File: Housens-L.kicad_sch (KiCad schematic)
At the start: 37 parts, among them J1 JTAG/SWD, J2 USB_C_2.0, SW1 RESET, U1 MCP1603, U2 BME280, U3 OPT3005, U4 STM32WB55CGUx, Y1 32MHz, Y2 32.768kHz

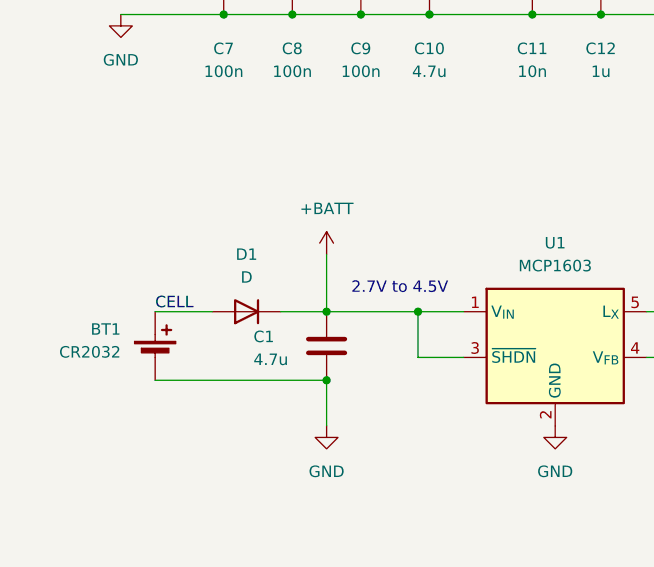
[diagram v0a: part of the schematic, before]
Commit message: Layout antenna
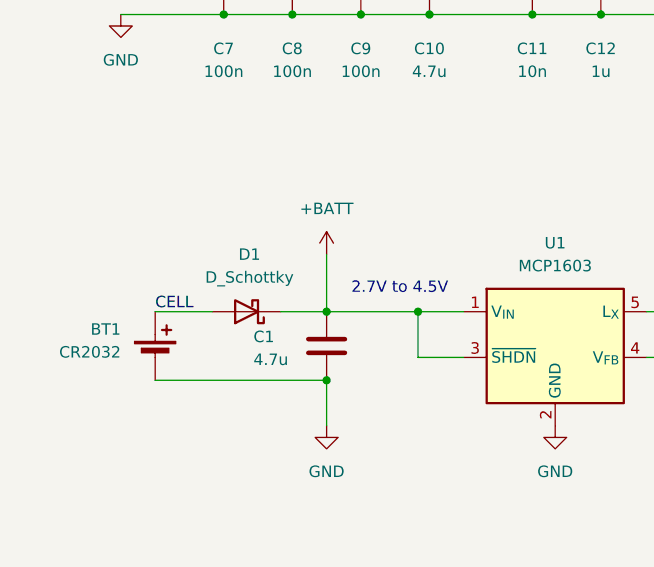
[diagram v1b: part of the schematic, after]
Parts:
- removed D1: D, Diode_SMD:D_0603_1608Metric, symbol Device:D
- added D1: D_Schottky, Diode_SMD:D_0603_1608Metric, symbol Device:D_Schottky
- Y1, Y2: footprint (none) -> Crystal:Crystal_SMD_2520-4Pin_2.5x2.0mm
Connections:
- net +BATT: now also D1.1 (K)
- net CELL: now also D1.2 (A)
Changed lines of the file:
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@@
+	)
+	(symbol
+		(lib_id "Device:D_Schottky")
+		(at 40.64 170.18 180)
+		(unit 1)
+		(exclude_from_sim no)
+		(in_bom yes)
+		(on_board yes)
+		(dnp no)
+		(fields_autoplaced yes)
+		(property "Reference" "D1"
+			(at 40.9575 163.83 0)
+			(effects
+				(font
+					(size 1.27 1.27)
+				)
+			)
+		)
+		(property "Value" "D_Schottky"
+			(at 40.9575 166.37 0)
+			(effects
+				(font
+					(size 1.27 1.27)
+				)
+			)
+		)
+		(property "Footprint" "Diode_SMD:D_0603_1608Metric"
+			(at 40.64 170.18 0)
+			(effects
+				(font
+					(size 1.27 1.27)
+				)
+				(hide yes)
+			)
+		)
+		(property "Datasheet" "~"
+			(at 40.64 170.18 0)
+			(effects
+				(font
+					(size 1.27 1.27)
+				)
+				(hide yes)
+			)
+		)
+		(property "Description" "Schottky diode"
+			(at 40.64 170.18 0)
+			(effects
+				(font
+					(size 1.27 1.27)
+				)
+				(hide yes)
+			)
+		)
+		(pin "2"
+		)
+		(pin "1"
+		)
+		(instances
+			(project ""
+				(path "/36bb4837-104c-4aa4-b300-0e6d0ff24db5"
+					(reference "D1")
+					(unit 1)
+				)
+			)
+		)
 	)
 	(symbol
@@
 	)
 	(symbol
-		(lib_id "Device:D")
-		(at 40.64 170.18 180)
-		(unit 1)
-		(exclude_from_sim no)
-		(in_bom yes)
-		(on_board yes)
-		(dnp no)
-		(fields_autoplaced yes)
-		(property "Reference" "D1"
-			(at 40.64 163.83 0)
-			(effects
-				(font
-					(size 1.27 1.27)
-				)
-			)
-		)
-		(property "Value" "D"
-			(at 40.64 166.37 0)
-			(effects
-				(font
-					(size 1.27 1.27)
-				)
-			)
-		)
-		(property "Footprint" "Diode_SMD:D_0603_1608Metric"
-			(at 40.64 170.18 0)
-			(effects
-				(font
-					(size 1.27 1.27)
-				)
-				(hide yes)
-			)
-		)
-		(property "Datasheet" "~"
-			(at 40.64 170.18 0)
-			(effects
-				(font
-					(size 1.27 1.27)
-				)
-				(hide yes)
-			)
-		)
-		(property "Description" "Diode"
-			(at 40.64 170.18 0)
-			(effects
-				(font
-					(size 1.27 1.27)
-				)
-				(hide yes)
-			)
-		)
-		(property "Sim.Device" "D"
-			(at 40.64 170.18 0)
-			(effects
-				(font
-					(size 1.27 1.27)
-				)
-				(hide yes)
-			)
-		)
-		(property "Sim.Pins" "1=K 2=A"
-			(at 40.64 170.18 0)
-			(effects
-				(font
-					(size 1.27 1.27)
-				)
-				(hide yes)
-			)
-		)
-		(pin "1"
-		)
-		(pin "2"
-		)
-		(instances
-			(project ""
-				(path "/36bb4837-104c-4aa4-b300-0e6d0ff24db5"
-					(reference "D1")
-					(unit 1)
-				)
-			)
-		)
-	)
-	(symbol
 		(lib_id "Device:C")
 		(at 38.1 133.35 0)
@@
 			)
 		)
-		(property "Footprint" ""
+		(property "Footprint" "Crystal:Crystal_SMD_2520-4Pin_2.5x2.0mm"
 			(at 24.13 82.55 0)
 			(effects
@@
 			)
 		)
-		(property "Footprint" ""
+		(property "Footprint" "Crystal:Crystal_SMD_2520-4Pin_2.5x2.0mm"
 			(at 24.13 54.61 0)
 			(effects
